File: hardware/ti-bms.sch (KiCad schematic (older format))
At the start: 64 parts, among them J1 Conn_02x03_Odd_Even, J2 Conn_01x02, J3 Conn_01x02, J4 Conn_01x02, J5 CAN_TERM, U1 Pico, U2 MCP2515-xST, U3 SN65HVD231, U4 TPS62160DGK, U5 MAX3485, U6 MAX3485, U7 MAX3485

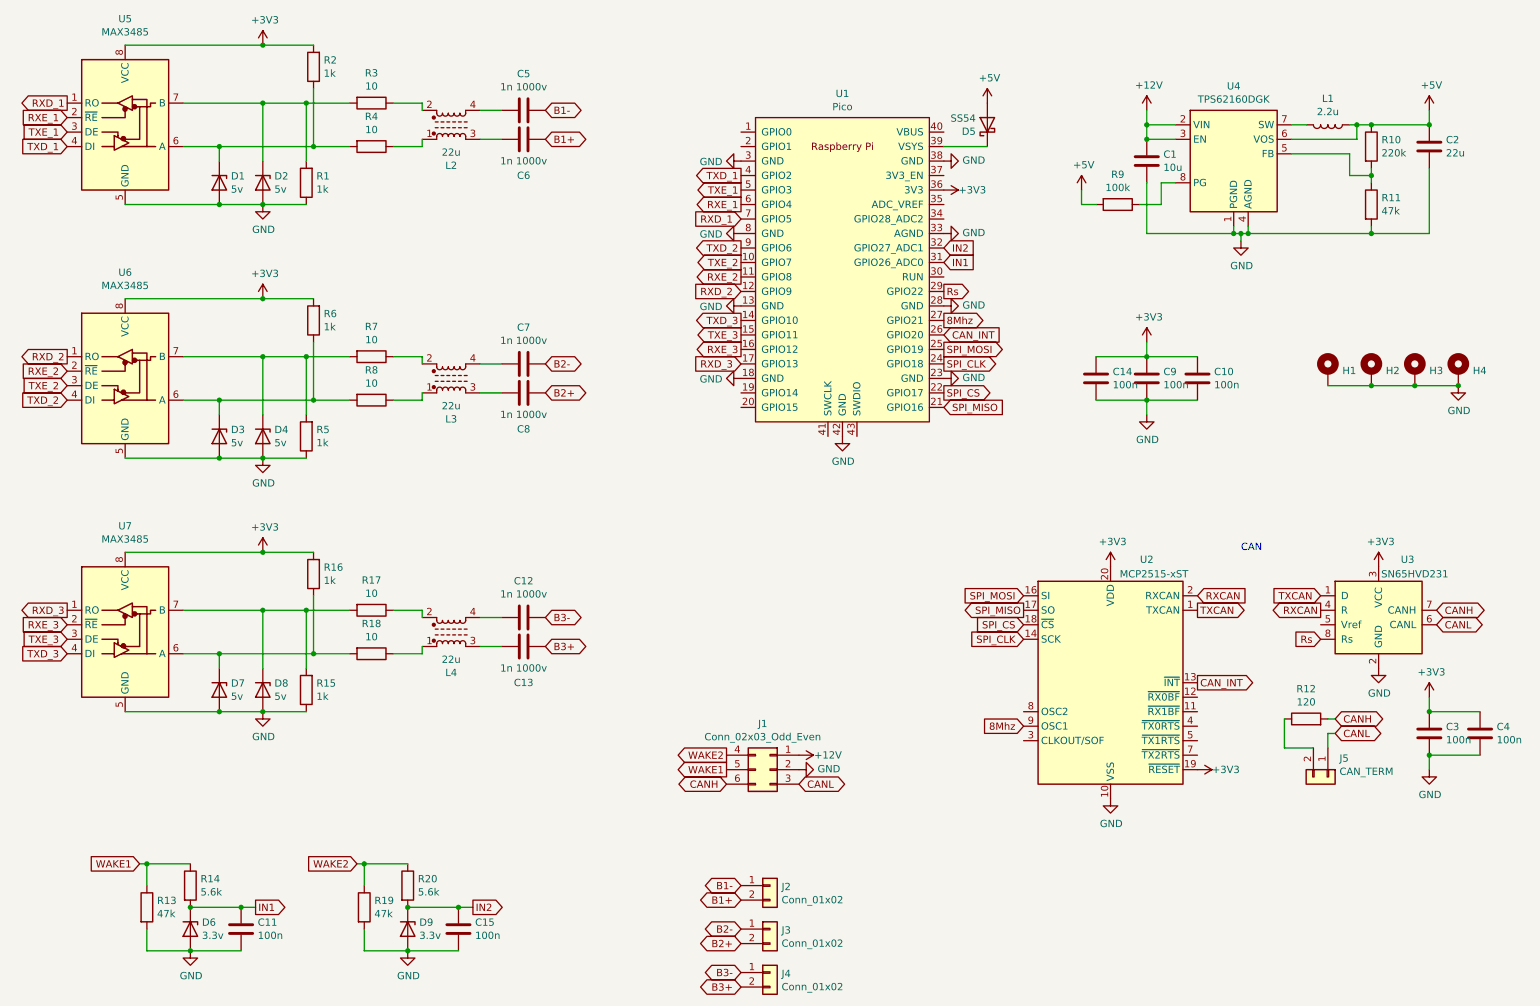
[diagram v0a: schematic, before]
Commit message: merge v3 improvements into v2
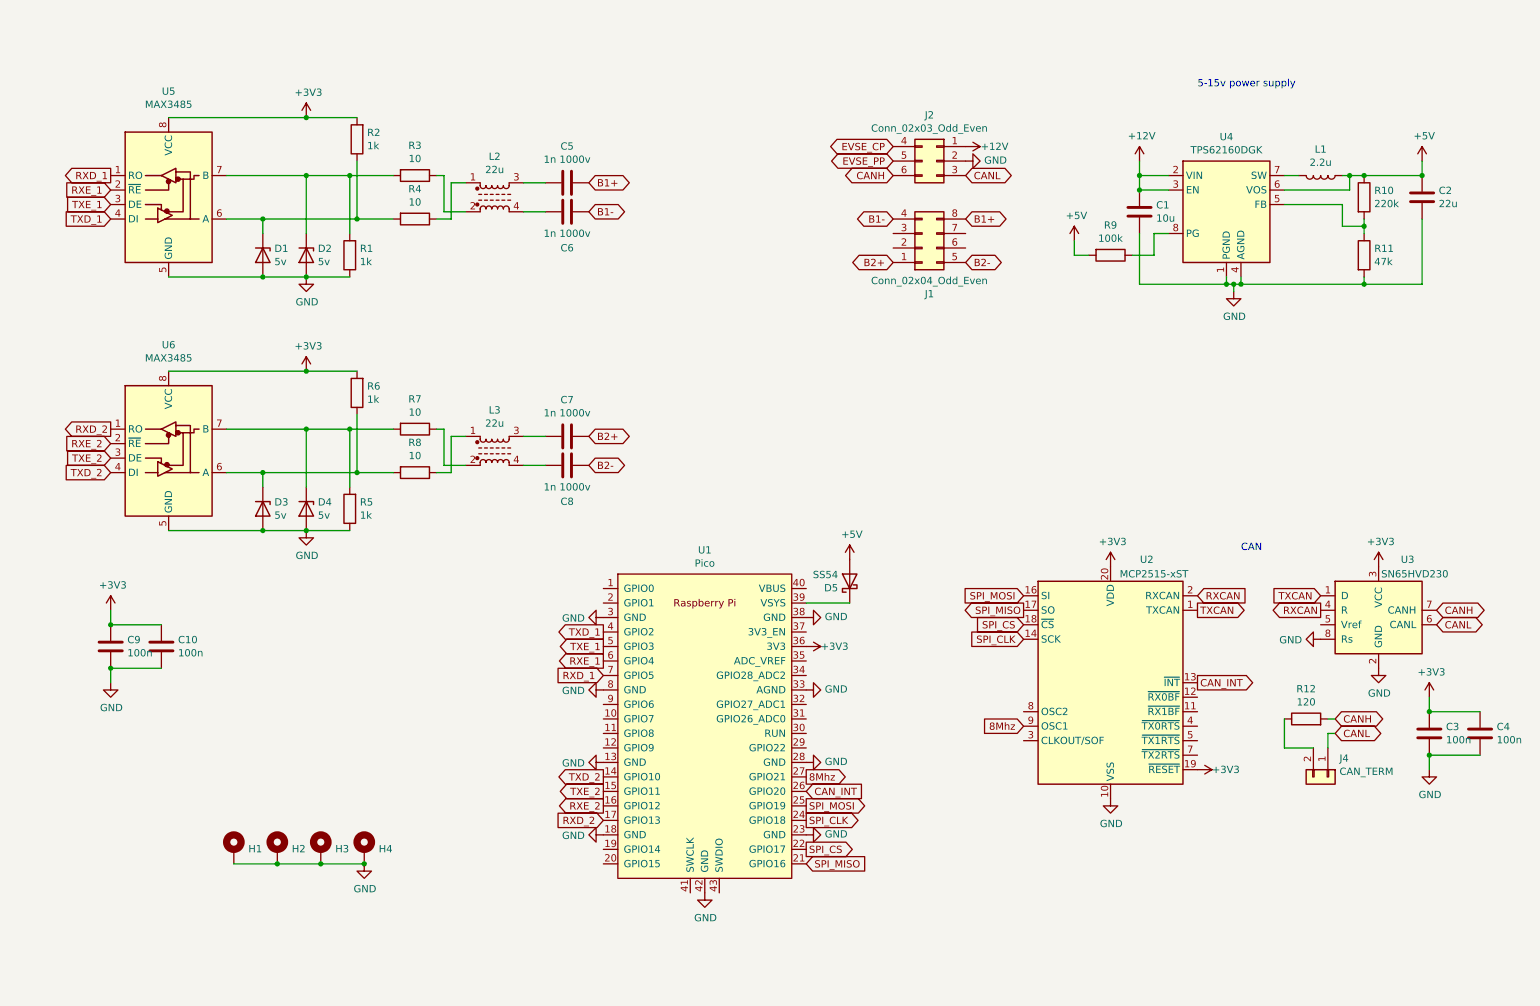
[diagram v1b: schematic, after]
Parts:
- removed C11, C14, C15: 100n, Capacitor_SMD:C_0603_1608Metric, symbol Device:C
- removed C12, C13: 1n 1000v, Capacitor_SMD:C_1206_3216Metric, symbol Device:C
- removed D6, D9: 3.3v, Diode_SMD:D_MiniMELF, symbol Device:D_Zener
- removed D7, D8: 5v, footprints:SOD882, symbol Device:D_Zener
- removed J2, J3, J4: Conn_01x02, Connector_Molex:Molex_Micro-Fit_3.0_43650-0200_1x02_P3.00mm_Horizontal, symbol Connector_Generic:Conn_01x02
- removed L4: 22u, footprints:ACT45B-101-2P-TL003, symbol Device:L_Core_Ferrite_Coupled_1324
- removed R13, R19: 47k, Resistor_SMD:R_0603_1608Metric, symbol Device:R
- removed R14, R20: 5.6k, Resistor_SMD:R_0603_1608Metric, symbol Device:R
- removed R15, R16: 1k, Resistor_SMD:R_0603_1608Metric, symbol Device:R
- removed R17, R18: 10, Resistor_SMD:R_0603_1608Metric, symbol Device:R
- removed U7: MAX3485, Package_SO:SOP-8_3.9x4.9mm_P1.27mm, symbol Interface_UART:MAX3485
- added J1: Conn_02x04_Odd_Even, Connector_Molex:Molex_Micro-Fit_3.0_43045-0800_2x04_P3.00mm_Horizontal, symbol Connector_Generic:Conn_02x04_Top_Bottom
- C2: LCSC C5672 -> C12891
- L1: footprint Inductor_SMD:L_Neosid_SMS-ME3015 -> footprints:1227ASH100MP2; LCSC C43389 -> C435389
- U3: value SN65HVD231 -> SN65HVD230; LCSC C129257 -> C12084
- renumbered J1 to J2, J5 to J4
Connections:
- net RXD_3 is gone; now on net RXD_2: U1.17 (GPIO13)
- net RXE_3 is gone; now on net RXE_2: U1.16 (GPIO12)
- net TXD_3 is gone; now on net TXD_2: U1.14 (GPIO10)
- net TXE_3 is gone; now on net TXE_2: U1.15 (GPIO11)
- net B1+: now also C5.1, J1.8 (Pin_8); no longer C6.1
- net B1-: now also C6.1, J1.4 (Pin_4); no longer C5.1
- net B2+: now also C7.1, J1.1 (Pin_1); no longer C8.1
- net B2-: now also C8.1, J1.5 (Pin_5); no longer C7.1
- net GND: now also U3.8 (Rs)
- net RXD_2: no longer U1.12 (GPIO9)
- net RXE_2: no longer U1.11 (GPIO8)
- net TXD_2: no longer U1.9 (GPIO6)
- net TXE_2: no longer U1.10 (GPIO7)
- net at L2.3: now also C5.2; no longer C6.2
- net at L2.4: now also C6.2; no longer C5.2
- net at L3.3: now also C7.2; no longer C8.2
- net at L3.4: now also C8.2; no longer C7.2
- net IN1: no longer names the net of U1.31 (GPIO26_ADC0)
- net IN2: no longer names the net of U1.32 (GPIO27_ADC1)
- net Rs: no longer names the net of U1.29 (GPIO22)
- net Rs: no longer U3.8 (Rs)
- net WAKE1 renamed EVSE_PP
- net WAKE2 renamed EVSE_CP
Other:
- note added: "5-15v power supply"
- moved on the sheet: C1, C10, C2, C5, C6, C7, C8, C9, D1, D2, D3, D4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
